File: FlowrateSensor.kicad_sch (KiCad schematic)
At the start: 21 parts, among them Q7 PMOS, Q8 BUK6M61-60PX, U6 TPS5405DR

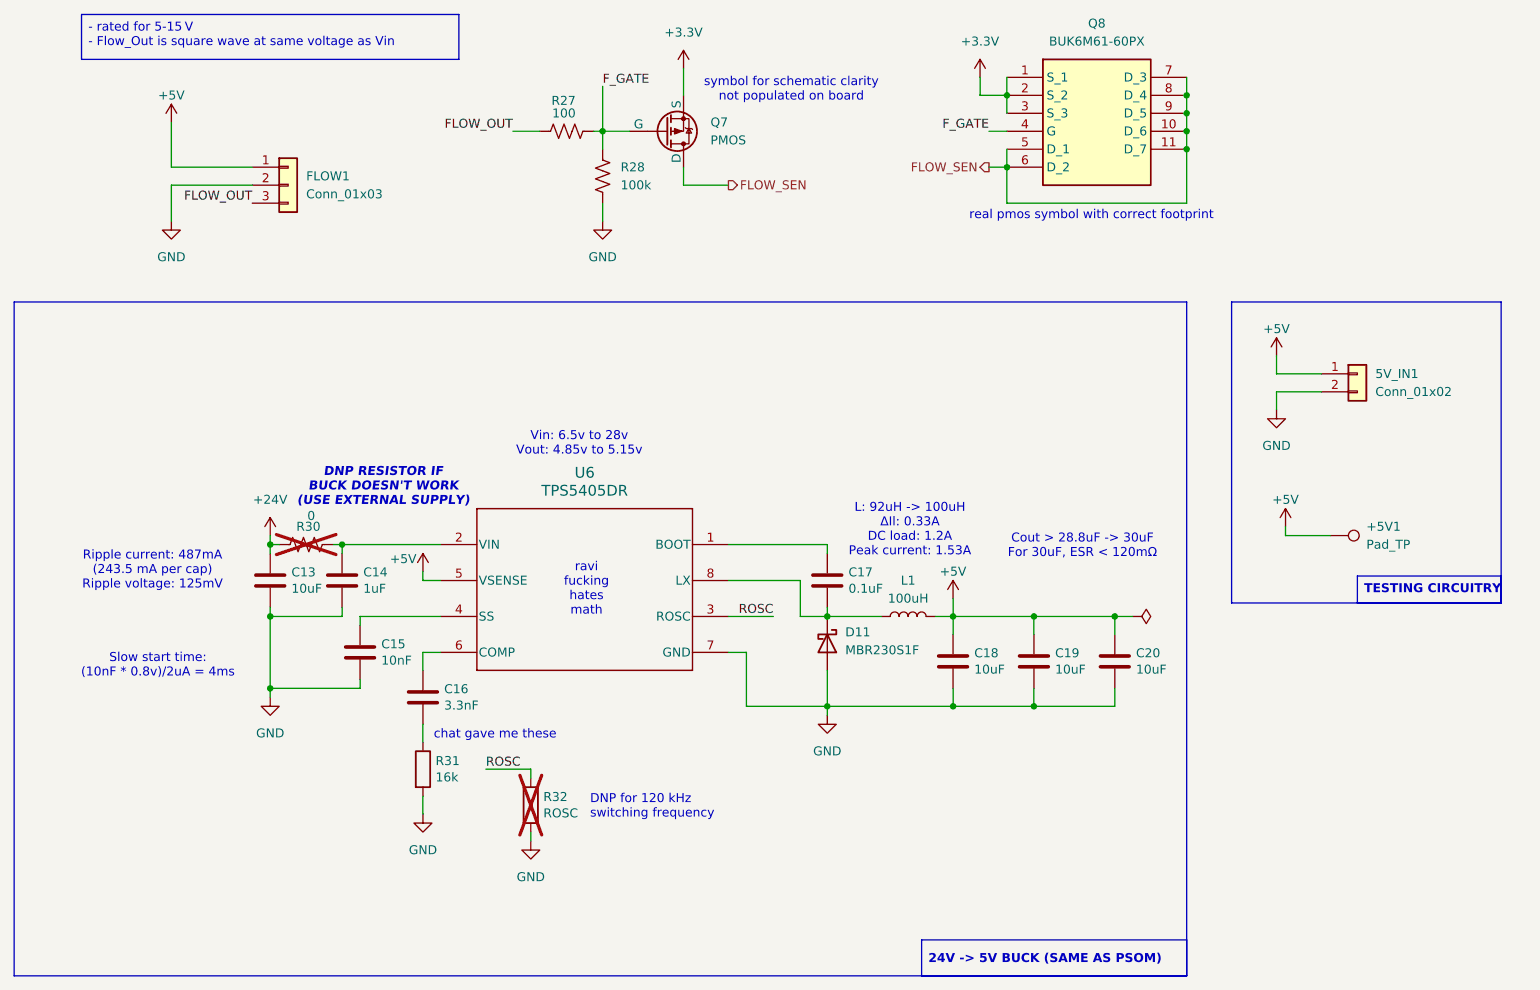
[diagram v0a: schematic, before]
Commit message: initial schem changes
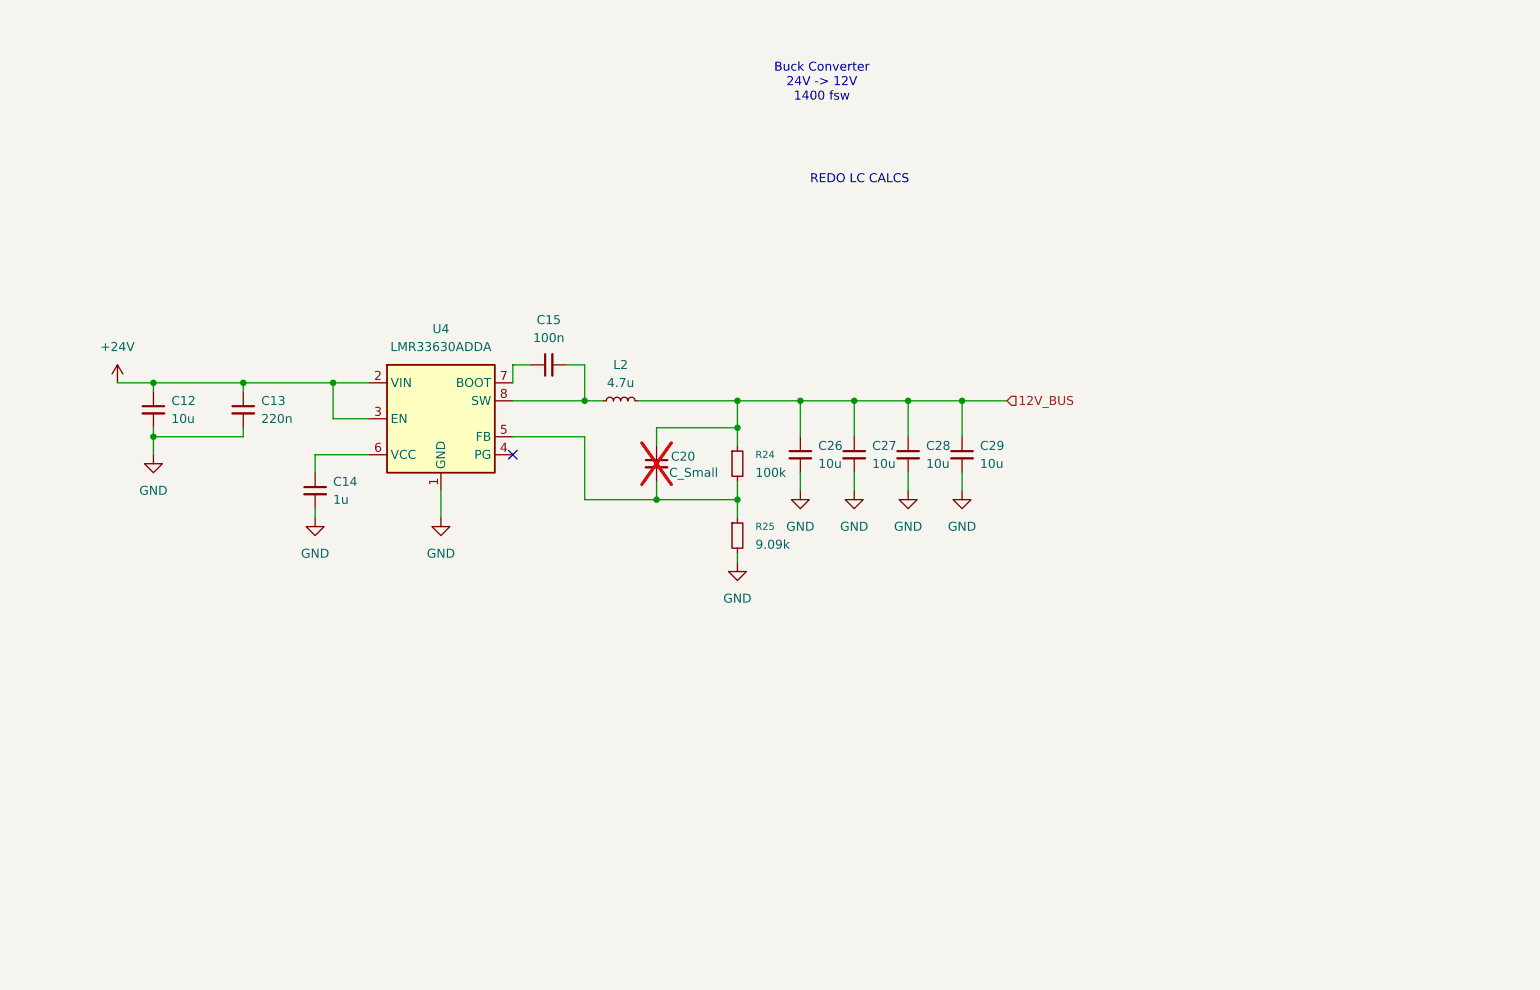
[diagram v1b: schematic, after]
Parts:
- removed +5V1: Pad_TP, UTSVT_Special:TestPoint_HEX_3mmID, symbol Connector:TestPoint
- removed 5V_IN1: Conn_01x02, UTSVT_Connectors:Molex_Nano-Fit_105309-xx02_1x02_P2.50mm_Vertical, symbol Connector_Generic:Conn_01x02
- removed C13, C18, C19, C20: 10uF, Capacitor_SMD:C_0805_2012Metric_Pad1.18x1.45mm_HandSolder, symbol Device:C
- removed C14: 1uF, Capacitor_SMD:C_0603_1608Metric_Pad1.08x0.95mm_HandSolder, symbol Device:C
- removed C15: 10nF, Capacitor_SMD:C_0603_1608Metric_Pad1.08x0.95mm_HandSolder, symbol Device:C
- removed C16: 3.3nF, Capacitor_SMD:C_0603_1608Metric_Pad1.08x0.95mm_HandSolder, symbol Device:C
- removed C17: 0.1uF, Capacitor_SMD:C_0603_1608Metric_Pad1.08x0.95mm_HandSolder, symbol Device:C
- removed D11: MBR230S1F, Diode_SMD:D_SOD-123F, symbol Device:D_Schottky
- removed FLOW1: Conn_01x03, Connector_Molex:Molex_Nano-Fit_105309-xx03_1x03_P2.50mm_Vertical, symbol Connector_Generic:Conn_01x03
- removed L1: 100uH, Inductor_SMD:L_Coilcraft_MSS1246-XXX, symbol Device:L
- removed Q7: PMOS, symbol Simulation_SPICE:PMOS
- removed Q8: BUK6M61-60PX, BUK6M61-60PX:BUK9M34100EX, symbol BUK6M61-60PX:BUK6M61-60PX
- removed R27: 100, Resistor_SMD:R_0603_1608Metric, symbol Device:R_US
- removed R28: 100k, Resistor_SMD:R_0603_1608Metric, symbol Device:R_US
- removed R30: 0, Resistor_SMD:R_0603_1608Metric, symbol Device:R_US
- removed R31: 16k, Resistor_SMD:R_0603_1608Metric_Pad0.98x0.95mm_HandSolder, symbol Device:R
- removed R32: ROSC, Resistor_SMD:R_0603_1608Metric_Pad0.98x0.95mm_HandSolder, symbol Device:R
- removed U6: TPS5405DR, UTSVT_Power:TPS5405DR, symbol utsvt_power:TPS5405DR
- added C12, C26, C27, C28, C29: 10u, Capacitor_SMD:C_0805_2012Metric_Pad1.18x1.45mm_HandSolder, symbol Device:C_Small
- added C13: 220n, Capacitor_SMD:C_0603_1608Metric_Pad1.08x0.95mm_HandSolder, symbol Device:C_Small
- added C14: 1u, Capacitor_SMD:C_0603_1608Metric_Pad1.08x0.95mm_HandSolder, symbol Device:C_Small
- added C15: 100n, Capacitor_SMD:C_0603_1608Metric_Pad1.08x0.95mm_HandSolder, symbol Device:C_Small
- added C20: C_Small, Capacitor_SMD:C_0603_1608Metric_Pad1.08x0.95mm_HandSolder, symbol Device:C_Small
- added L2: 4.7u, easyeda2kicad:IND-SMD_L5.0-W5.0, symbol Device:L_Small
- added R24: 100k, Resistor_SMD:R_0603_1608Metric_Pad0.98x0.95mm_HandSolder, symbol Device:R_Small
- added R25: 9.09k, Resistor_SMD:R_0603_1608Metric_Pad0.98x0.95mm_HandSolder, symbol Device:R_Small
- added U4: LMR33630ADDA, Package_SO:Texas_HSOP-8-1EP_3.9x4.9mm_P1.27mm_ThermalVias, symbol Regulator_Switching:LMR33630ADDA
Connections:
- net +24V: now also C12.1, C13.1, U4.2 (VIN), U4.3 (EN)
- net GND: now also C12.2, C13.2, C14.2, C26.2, C27.2, C28.2, C29.2, R25.2, U4.1 (GND), U4.9 (GND)
- new net: C14.1, U4.6 (VCC)
- new net: C15.2, L2.1, U4.8 (SW)
- new net: C20.2, R24.2, R25.1, U4.5 (FB)
- new net: C15.1, U4.7 (BOOT)
- new net 12V_BUS: C20.1, C26.1, C27.1, C28.1, C29.1, L2.2, R24.1
- no-connect marks 0 -> 1
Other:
- note added: "Buck Converter 24V -> 12V 1400 fsw"
- note added: "REDO LC CALCS"
- note removed: "Cout > 28.8uF -> 30uF For 30uF, ESR < 120mΩ"
- note removed: "DNP RESISTOR IF BUCK DOESN'T WORK (USE EXTERNAL SUPPLY)"
- note removed: "DNP for 120 kHz switching frequency"
- note removed: "L: 92uH -> 100uH ΔIl: 0.33A DC load: 1.2A Peak current: 1.53A"
- note removed: "Ripple current: 487mA (243.5 mA per cap) Ripple voltage: 125mV"
- note removed: "Slow start time: (10nF * 0.8v)/2uA = 4ms"
- note removed: "Vin: 6.5v to 28v Vout: 4.85v to 5.15v"
- note removed: "chat gave me these"
- note removed: "ravi fucking hates math"
- note removed: "real pmos symbol with correct footprint"
- note removed: "symbol for schematic clarity not populated on board"
